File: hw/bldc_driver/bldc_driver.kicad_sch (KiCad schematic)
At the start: 48 parts, among them J1 430450412, J2 B4B-EH-A(LF)(SN), J3 B4B-EH-A(LF)(SN), J4 1733583, SW1 BTSA-N-P-1, U1 CH32V30xRxTx, U14 SN65HVD230, U8 TPS54202DDC, Y1 Crystal_GND24

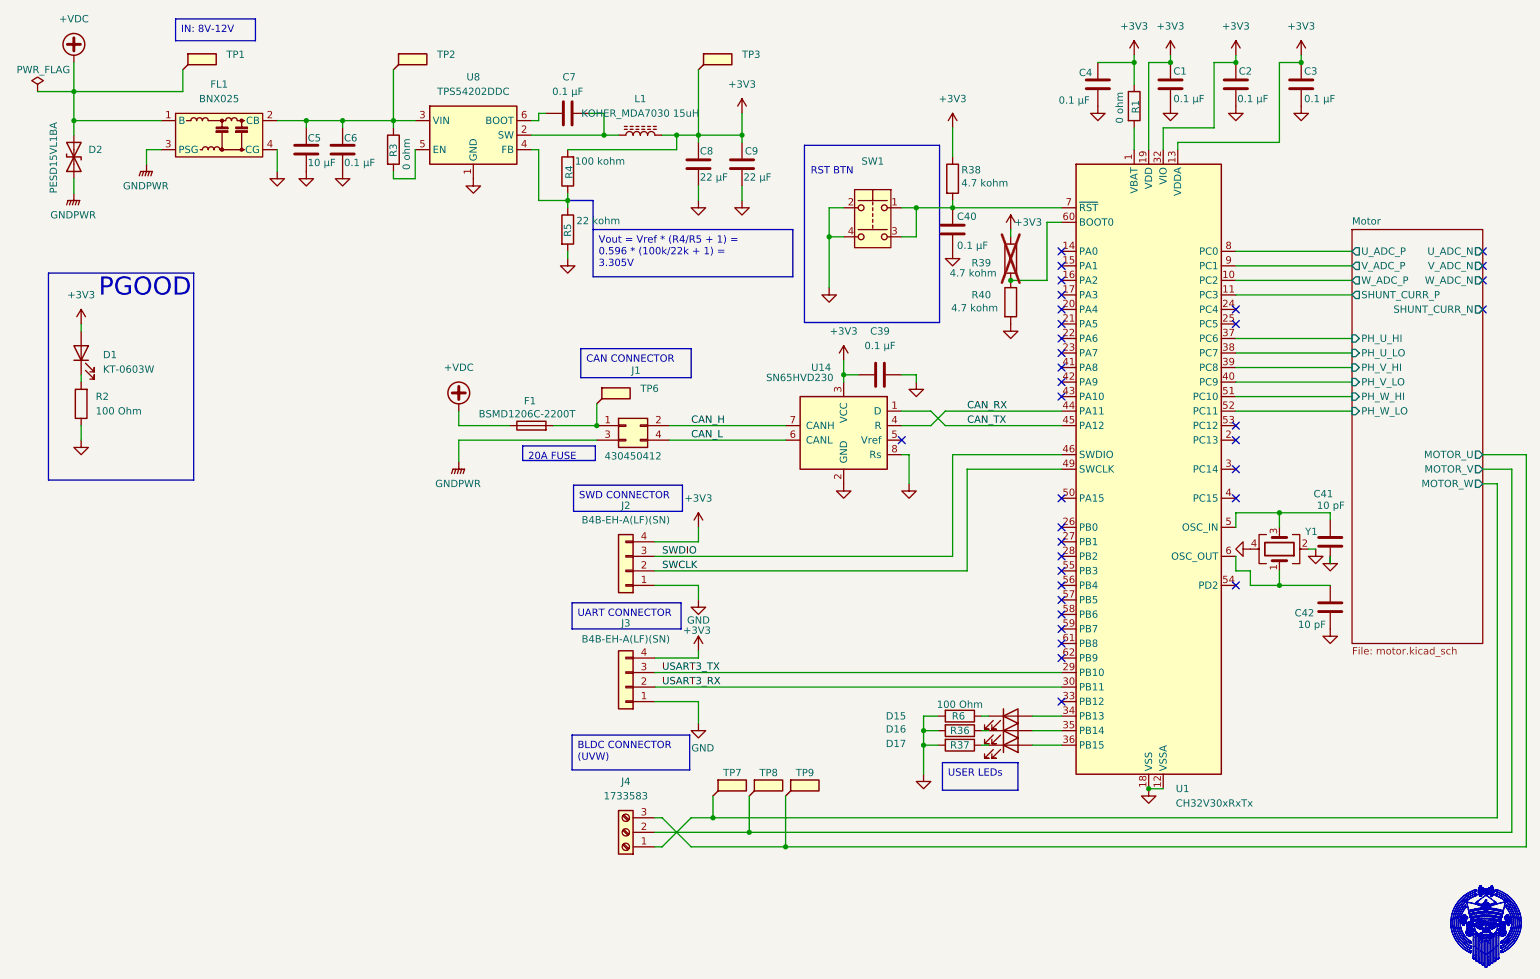
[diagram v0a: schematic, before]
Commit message: before reroute
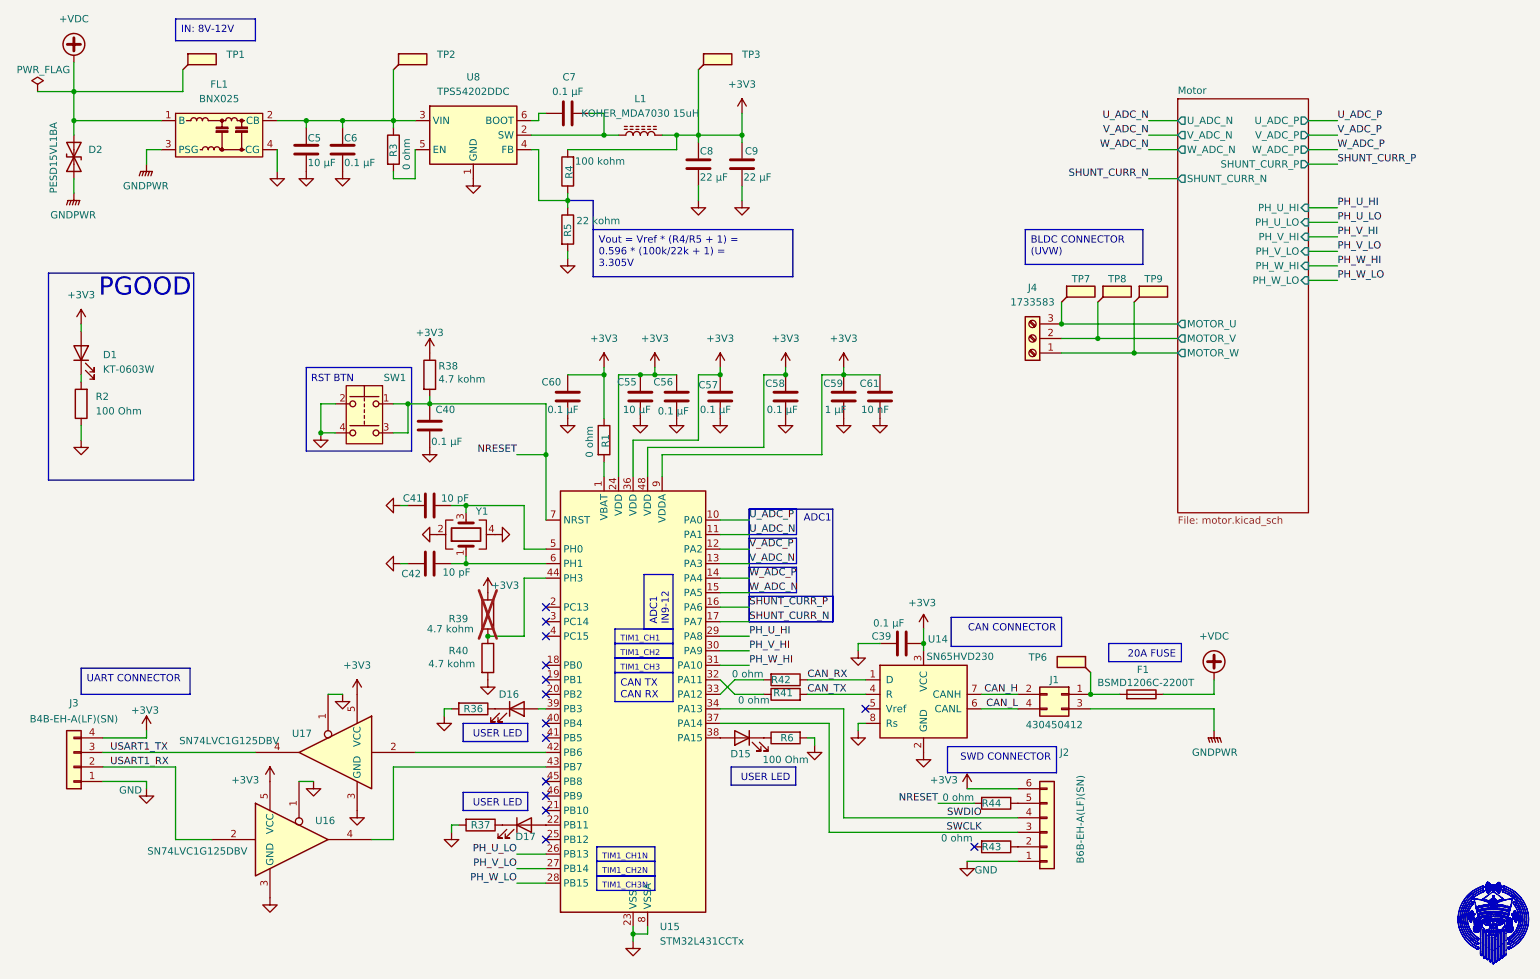
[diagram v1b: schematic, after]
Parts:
- removed C1, C2, C3, C4: 0.1 µF, Capacitor_SMD:C_0805_2012Metric_Pad1.18x1.45mm_HandSolder, symbol #inventree:CL21B104KBCNNNC
- removed U1: CH32V30xRxTx, Package_QFP:LQFP-64_10x10mm_P0.5mm, symbol MCU_WCH_CH32V3:CH32V30xRxTx
- added C55: 10 µF, Capacitor_SMD:C_0805_2012Metric_Pad1.18x1.45mm_HandSolder, symbol #inventree:CL21A106KOQNNNE
- added C56, C57, C58, C60: 0.1 µF, Capacitor_SMD:C_0805_2012Metric_Pad1.18x1.45mm_HandSolder, symbol #inventree:CL21B104KBCNNNC
- added C59: 1 µF, Capacitor_SMD:C_0805_2012Metric_Pad1.18x1.45mm_HandSolder, symbol #inventree:CL21B104KBCNNNC
- added C61: 10 nF, Capacitor_SMD:C_0805_2012Metric_Pad1.18x1.45mm_HandSolder, symbol #inventree:CL21B104KBCNNNC
- added R41, R42, R43, R44: 0 ohm, Resistor_SMD:R_0603_1608Metric_Pad0.98x0.95mm_HandSolder, symbol #inventree:RC0603FR-070RL
- added U15: STM32L431CCTx, Package_QFP:LQFP-48_7x7mm_P0.5mm, symbol MCU_ST_STM32L4:STM32L431CCTx
- added U16, U17: SN74LVC1G125DBV, Package_TO_SOT_SMD:SOT-23-5_HandSoldering, symbol 74xGxx:SN74LVC1G125DBV
- J2: value B4B-EH-A(LF)(SN) -> B6B-EH-A(LF)(SN); footprint Connector_JST:JST_EH_B4B-EH-A_1x04_P2.50mm_Vertical -> Connector_JST:JST_EH_B6B-EH-A_1x06_P2.50mm_Vertical; symbol Connector_Generic:Conn_01x04 -> Connector_Generic:Conn_01x06
- R4: footprint Resistor_SMD:R_0201_0603Metric_Pad0.64x0.40mm_HandSolder -> Resistor_SMD:R_0603_1608Metric_Pad0.98x0.95mm_HandSolder
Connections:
- net +3V3: now also J2.6 (Pin_6), C55.1, C56.2, C57.2, C58.2, C59.2, C60.2, C61.2, U15.24 (VDD), U15.36 (VDD), U15.48 (VDD), U15.9 (VDDA), U16.5 (VCC), U17.5 (VCC); no longer J2.4 (Pin_4)
- net CAN_RX: now also U14.1 (D), R42.1; no longer U14.4 (R)
- net CAN_TX: now also U14.4 (R), R41.2; no longer U14.1 (D)
- net GND: now also C41.1, C42.1, C55.2, C56.1, C57.1, C58.1, C59.1, C60.1, C61.1, U15.23 (VSS), U15.35 (VSS), U15.47 (VSS), U15.8 (VSSA), U16.1, U16.3 (GND), U17.1, U17.3 (GND); no longer C41.2, C42.2
- net Motor/MOTOR_U: now also TP7.1; no longer TP9.1
- net Motor/MOTOR_W: now also TP9.1; no longer TP7.1
- net SWCLK: now also J2.3 (Pin_3), U15.37 (PA14); no longer J2.2 (Pin_2)
- net SWDIO: now also J2.4 (Pin_4), U15.34 (PA13); no longer J2.3 (Pin_3)
- net at R1.2: now also U15.1 (VBAT)
- net at D15.2 (A): now also U15.38 (PA15)
- net at D16.2 (A): now also U15.39 (PB3)
- net at D17.2 (A): now also U15.22 (PB11)
- net at Y1.3: now also C41.2, U15.5 (PH0); no longer C41.1
- net at Y1.1: now also C42.2, U15.6 (PH1); no longer C42.1
- net at R39.2, R40.1: now also U15.44 (PH3)
- net NRESET: now reaches C40.1, R38.2, SW1.1, SW1.3
- net NRESET: now also R44.2, U15.7 (NRST)
- net USART3_RX renamed USART1_RX
- net USART1_RX: now also U16.2
- net USART3_TX renamed USART1_TX
- net USART1_TX: now also U17.4
- new net: J2.2 (Pin_2), R43.1
- new net: U15.43 (PB7), U16.4
- new net: R42.2, U15.33 (PA12)
- new net: R41.1, U15.32 (PA11)
- new net: J2.5 (Pin_5), R44.1
- new net: U15.42 (PB6), U17.2
- new net PH_U_HI: U15.29 (PA8)
- new net PH_U_LO: U15.26 (PB13)
- new net PH_V_HI: U15.30 (PA9)
- new net PH_V_LO: U15.27 (PB14)
- new net PH_W_HI: U15.31 (PA10)
- new net PH_W_LO: U15.28 (PB15)
- new net SHUNT_CURR_N: U15.17 (PA7)
- new net SHUNT_CURR_P: U15.16 (PA6)
- new net U_ADC_N: U15.11 (PA1)
- new net U_ADC_P: U15.10 (PA0)
- new net V_ADC_N: U15.13 (PA3)
- new net V_ADC_P: U15.12 (PA2)
- new net W_ADC_N: U15.15 (PA5)
- new net W_ADC_P: U15.14 (PA4)
- no-connect marks 35 -> 14
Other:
- note added: "ADC1"
- moved on the sheet: C39, C40, C41, C42, D15, D16, D17, F1, J1, J3, J4, R1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
